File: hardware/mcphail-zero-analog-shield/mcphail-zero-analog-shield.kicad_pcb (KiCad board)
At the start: 2 copper layers, 80.6 x 56.6 mm, 143 parts, among them J1 INSECT DETECTION, J2 EMITTERS, J3 BREAKOUT, J4 MICRO SD, J5 MICRO USB, J6 PROG/BOOT, J7 FONA 808, J8 INPUT 6V-9V, J9 JST PH, U1 MCP6004, U10 BUCK-BOOST 5V TPS63060, U11 MCP1703, U2 MCP6004, U3 TLV274, U4 MCP6001, U5 ADS1118, U6 ATSAMD21G18A, U7 24AA1025 EEPROM, U8 MCP7940N RTC, U9 MCP73871, X1 16MHz, X2 32.768kHz

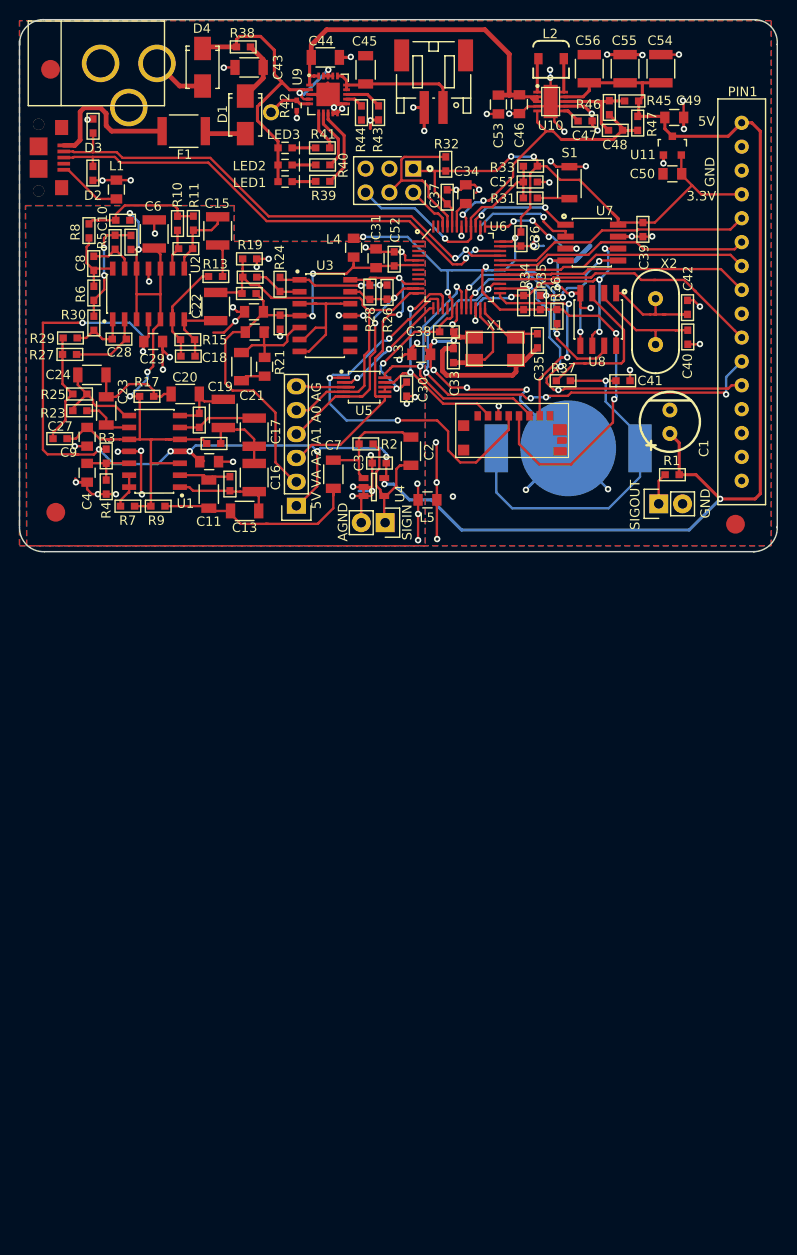
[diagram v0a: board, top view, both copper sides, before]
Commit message: Only comps we need left on board. Needs routed.
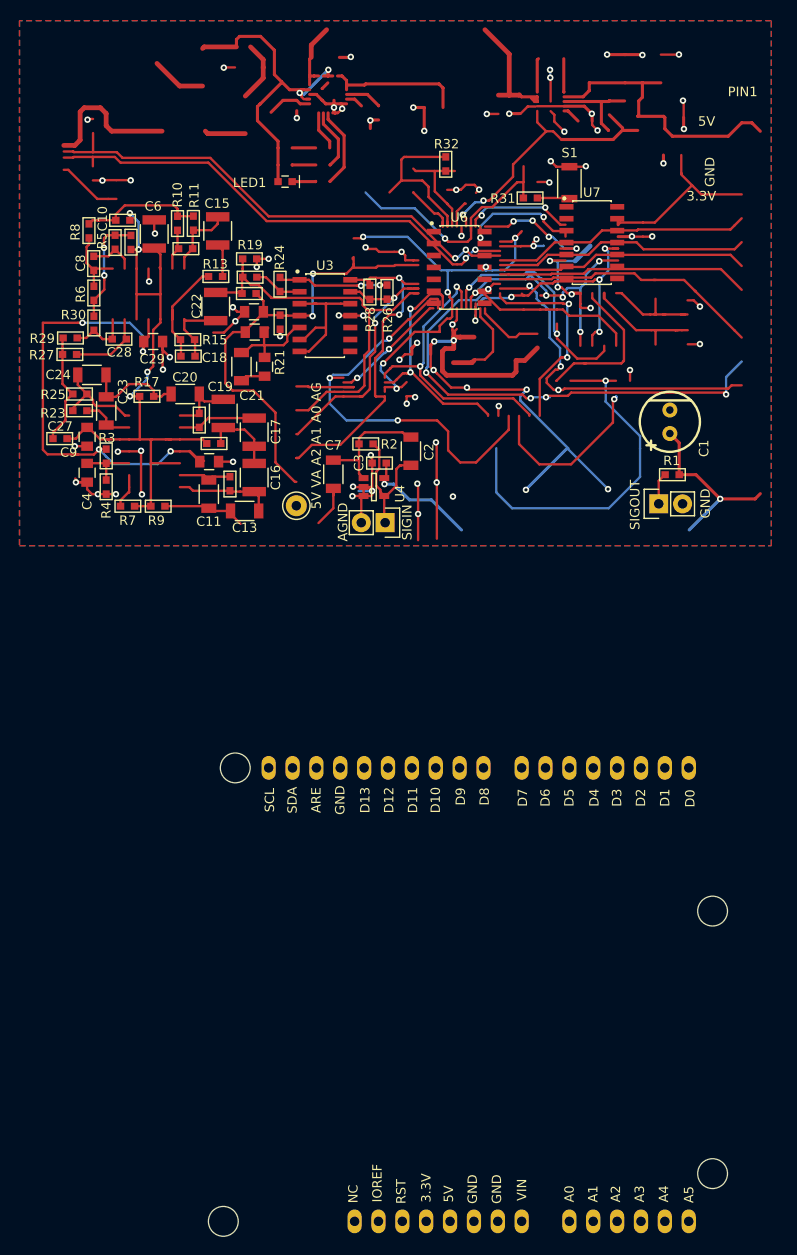
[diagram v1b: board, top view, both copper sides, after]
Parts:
- removed BAT1: 3V, Wickerlib:BATT-HOLDER-CR1220-BK-916
- removed C30, C36, C37, C38, C39, C47, C51, C52: 100nF, Wickerlib:RLC-0603-SMD
- removed C31, C46, C53: 10uF, Wickerlib:RLC-0805-SMD
- removed C33, C35: 22pF, Wickerlib:RLC-0603-SMD
- removed C34, C49, C50: 1uF, Wickerlib:RLC-0805-SMD
- removed C40, C42: 2pF, Wickerlib:RLC-0603-SMD
- removed C41: 100pF, Wickerlib:RLC-0603-SMD
- removed C43, C44, C45: 4.7uF, Wickerlib:RLC-1206-SMD
- removed C48: 10pF, Wickerlib:RLC-0603-SMD
- removed C54, C55, C56: 22uF, Wickerlib:RLC-1210-SMD
- removed D1, D4: 20V 1A, Wickerlib:DIODE-SMA
- removed D2, D3: CG0603MLC-05E, Wickerlib:RLC-0603-SMD
- removed F1: 500mA, Wickerlib:RLC-1812-SMD
- removed FID1, FID2, FID3: FIDUCIAL, Wickerlib:FIDUCIAL-2MM
- removed J4: MICRO SD, Wickerlib:CONN-SD-MICRO-MOLEX-0475710001
- removed J5: MICRO USB, Wickerlib:CONN-USB-MICRO-B-AMPHENOL-10118193-0001LF
- removed J6: PROG/BOOT, Wickerlib:CONN-HEADER-STRAIGHT-P2.54MM-2x03
- removed J7: FONA 808, Wickerlib:BREAKOUT-ADAFRUIT-FONA808-CELL-GPS
- removed J8: INPUT 6V-9V, Wickerlib:CONN-BARREL-JACK-2.5x5.5MM-TH
- removed J9: JST PH, Wickerlib:CONN-JST-S2B-PH-SM4-TB
- removed L1, L3, L4, L5: FERRITE, Wickerlib:RLC-0805-SMD
- removed L2: 1uH 3.3A, Wickerlib:1226AS-H-1R0N
- removed LED2, LED3: AMBER, Wickerlib:LED-0603-SMD
- removed R33, R36: 10K, Wickerlib:RLC-0603-SMD
- removed R34, R35, R43: 2K, Wickerlib:RLC-0603-SMD
- removed R37: 1K, Wickerlib:RLC-0603-SMD
- removed R38: 0 ohm, Wickerlib:RLC-0603-SMD
- removed R39, R40, R41: 470, Wickerlib:RLC-0603-SMD
- removed R42: NTC 10K, Wickerlib:RLC-0402-SMD
- removed R44: 100K, Wickerlib:RLC-0603-SMD
- removed R45, R47: 1M, Wickerlib:RLC-0603-SMD
- removed R46: 111K, Wickerlib:RLC-0603-SMD
- removed U1, U2: MCP6004, Wickerlib:SOIC-14-3.9x8.7MM-P1.27MM
- removed U11: MCP1703, Wickerlib:SOT-23-3
- removed U5: ADS1118, Wickerlib:MSOP-10-3x3MM-P0.5MM
- removed U8: MCP7940N RTC, Wickerlib:SOIC-8-3.9x4.9MM-P1.27MM
- removed U9: MCP73871, Wickerlib:QFN-20-1EP-4x4MM_P0.5MM
- removed W1: TEST_1P, Wickerlib:HOLE-PLATED-40MIL
- removed X1: 16MHz, Wickerlib:CRYSTAL-CTS-4SMD
- removed X2: 32.768kHz, Wickerlib:CRYSTAL-HC49-TH
- J3: value BREAKOUT -> VREF; footprint Wickerlib:CONN-HEADER-STRAIGHT-P2.54MM-1x06 -> Wickerlib:CONN-HEADER-STRAIGHT-P2.54MM-1x01
- R31: value 330 -> 0 ohm
- R32: value 1K -> 220
- U10: value BUCK-BOOST 5V TPS63060 -> ARDUINO-101-SHIELD; footprint Wickerlib:WSON-10-1EP -> Wickerlib:ARDUINO-UNO-SHIELD
- U6: value ATSAMD21G18A -> MCP6004; footprint Wickerlib:TQFP-48_7x7mm_Pitch0.5mm -> Wickerlib:SOIC-14-3.9x8.7MM-P1.27MM
- U7: value 24AA1025 EEPROM -> MCP6004; footprint Wickerlib:SOIC-8-3.9x4.9MM-P1.27MM -> Wickerlib:SOIC-14-3.9x8.7MM-P1.27MM
- moved U10 131.1 mm to (31.0, 172.6), turned to 0 degrees
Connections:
- net /Photodiode Signal Input Conditioning/PHOTO_K renamed /PHOTO_K
- C10 pad 2: /Photodiode Signal Input Conditioning/VREF -> /VREF
- C14 pad 2: AGND -> GND
- C18 pad 1: /Photodiode Signal Input Conditioning/LINE_IN -> /LINE_IN
- C22 pad 2: /Photodiode Signal Input Conditioning/LINE_IN -> /LINE_IN
- C25 pad 1: /VDDANA -> +3V3
- C25 pad 2: AGND -> GND
- C26 pad 1: /VDDANA -> +3V3
- C26 pad 2: AGND -> GND
- C27 pad 2: /Photodiode Signal Input Conditioning/VREF -> /VREF
- C29 pad 2: AGND -> GND
- C3 pad 2: AGND -> GND
- C4 pad 2: AGND -> GND
- C5 pad 2: /Photodiode Signal Input Conditioning/VREF -> /VREF
- C6 pad 1: /Photodiode Signal Input Conditioning/VREF -> /VREF
- C6 pad 2: AGND -> GND
- C9 pad 1: /Photodiode Signal Input Conditioning/VREF -> /VREF
- C9 pad 2: AGND -> GND
- J1 pad 2: AGND -> GND
- J3 pad 1: +5V -> /VREF
- LED1 pad 2: VIN -> Net-(LED1-Pad2)
- R14 pad 2: /Photodiode Signal Input Conditioning/VREF -> /VREF
- R15 pad 1: /Photodiode Signal Input Conditioning/LINE_IN -> /LINE_IN
- R17 pad 2: /Photodiode Signal Input Conditioning/VREF -> /VREF
- R18 pad 1: /VDDANA -> +3V3
- R19 pad 2: AGND -> GND
- R20 pad 1: /VDDANA -> +3V3
- R31 pad 1: /Microcontroller/~RESET -> +3V3
- R32 pad 1: +3V3 -> Net-(LED1-Pad1)
- R32 pad 2: /Microcontroller/SWCLK -> GND
- R4 pad 2: AGND -> GND
- R7 pad 1: /Photodiode Signal Input Conditioning/VREF -> /VREF
- R9 pad 2: /Photodiode Signal Input Conditioning/VREF -> /VREF
- S1 pad 1: Net-(R31-Pad2) -> Net-(S1-Pad1)
- U3 pad 11: AGND -> GND
- U3 pad 4: /VDDANA -> +3V3
- U4 pad 2: AGND -> GND
- U4 pad 3: AGND -> GND
- U6 pad 1: (no net) -> Net-(C13-Pad1)
- U6 pad 10: /A2 -> /VREF
- U6 pad 11: /A1 -> GND
- U6 pad 12: /A0 -> Net-(C4-Pad1)
- U6 pad 13: /Microcontroller/D4_CS -> Net-(R7-Pad2)
- U6 pad 14: /Microcontroller/SCLK -> Net-(R7-Pad2)
- U6 pad 2: (no net) -> Net-(C11-Pad1)
- U6 pad 3: (no net) -> /VREF
- U6 pad 4: (no net) -> +5V
- U6 pad 5: AGND -> /VREF
- U6 pad 6: /VDDANA -> Net-(C8-Pad2)
- U6 pad 7: (no net) -> Net-(C8-Pad1)
- U6 pad 8: (no net) -> Net-(C12-Pad1)
- U6 pad 9: (no net) -> Net-(C12-Pad2)
- U7 pad 1: /Microcontroller/EEPROM_ADD0 -> Net-(C28-Pad1)
- U7 pad 2: /Microcontroller/EEPROM_ADD1 -> Net-(C28-Pad2)
- U7 pad 3: /Microcontroller/EEPROM_ADD2 -> /VREF
- U7 pad 4: GND -> +5V
- U7 pad 5: /Microcontroller/SDA -> /VREF
- U7 pad 6: /Microcontroller/SCL -> Net-(C17-Pad1)
- U7 pad 7: GND -> Net-(C19-Pad1)
- U7 pad 8: +3V3 -> Net-(C24-Pad1)
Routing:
- net (no net): track 0.00 -> 967.4 mm, vias 1 -> 102
- net /VREF: track 0.00 -> 83.4 mm, vias 0 -> 6
- net AGND: track 75.7 -> 0.00 mm, vias 32 -> 0
- net +3V3: track 152.2 -> 76.8 mm, vias 10 -> 3
- net +5V: track 205.6 -> 132.0 mm, vias 9 -> 7
- net Net-(C12-Pad2): track 4.39 -> 74.0 mm, vias 0 -> 5
- net /Photodiode Signal Input Conditioning/VREF: track 69.5 -> 0.00 mm, vias 4 -> 0
- net GND: track 167.8 -> 111.3 mm, vias 53 -> 27
- net /Microcontroller/D-: track 54.6 -> 0.00 mm, vias 2 -> 0
- net /Microcontroller/D+: track 53.1 -> 0.00 mm, vias 2 -> 0
- net /Microcontroller/FONA_PS: track 52.2 -> 0.00 mm, vias 5 -> 0
- net /VDDANA: track 50.2 -> 0.00 mm, vias 2 -> 0
- net /Microcontroller/SCLK: track 45.9 -> 0.00 mm, vias 3 -> 0
- net Net-(BAT1-Pad1): track 38.7 -> 0.00 mm, vias 1 -> 0
- net /Input Power/VCC: track 38.3 -> 0.00 mm
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- removed copper zone on B.Cu, net AGND
- removed copper zone on F.Cu, net AGND
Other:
- board outline removed
